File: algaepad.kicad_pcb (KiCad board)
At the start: 2 copper layers, 10.6 x 5.5 mm, 64 parts, among them SW1 SW_Push, SW10 SW_Push, SW11 SW_Push, SW12 SW_Push, SW13 SW_Push, SW14 SW_Push, SW15 SW_Push, SW16 SW_Push, SW17 SW_Push, SW18 SW_Push, SW19 SW_Push, SW2 SW_Push, SW20 SW_Push, SW21 SW_Push, SW22 SW_Push, SW23 SW_Push, SW24 SW_Push, SW25 SW_Push, SW26 SW_Push, SW27 SW_Push, SW28 SW_Push, SW29 SW_Push, SW3 SW_Push, SW30 SW_Push, SW31 SW_Push, SW32 SW_Push, SW4 SW_Push, SW5 SW_Push, SW6 SW_Push, SW7 SW_Push, SW8 SW_Push, SW9 SW_Push

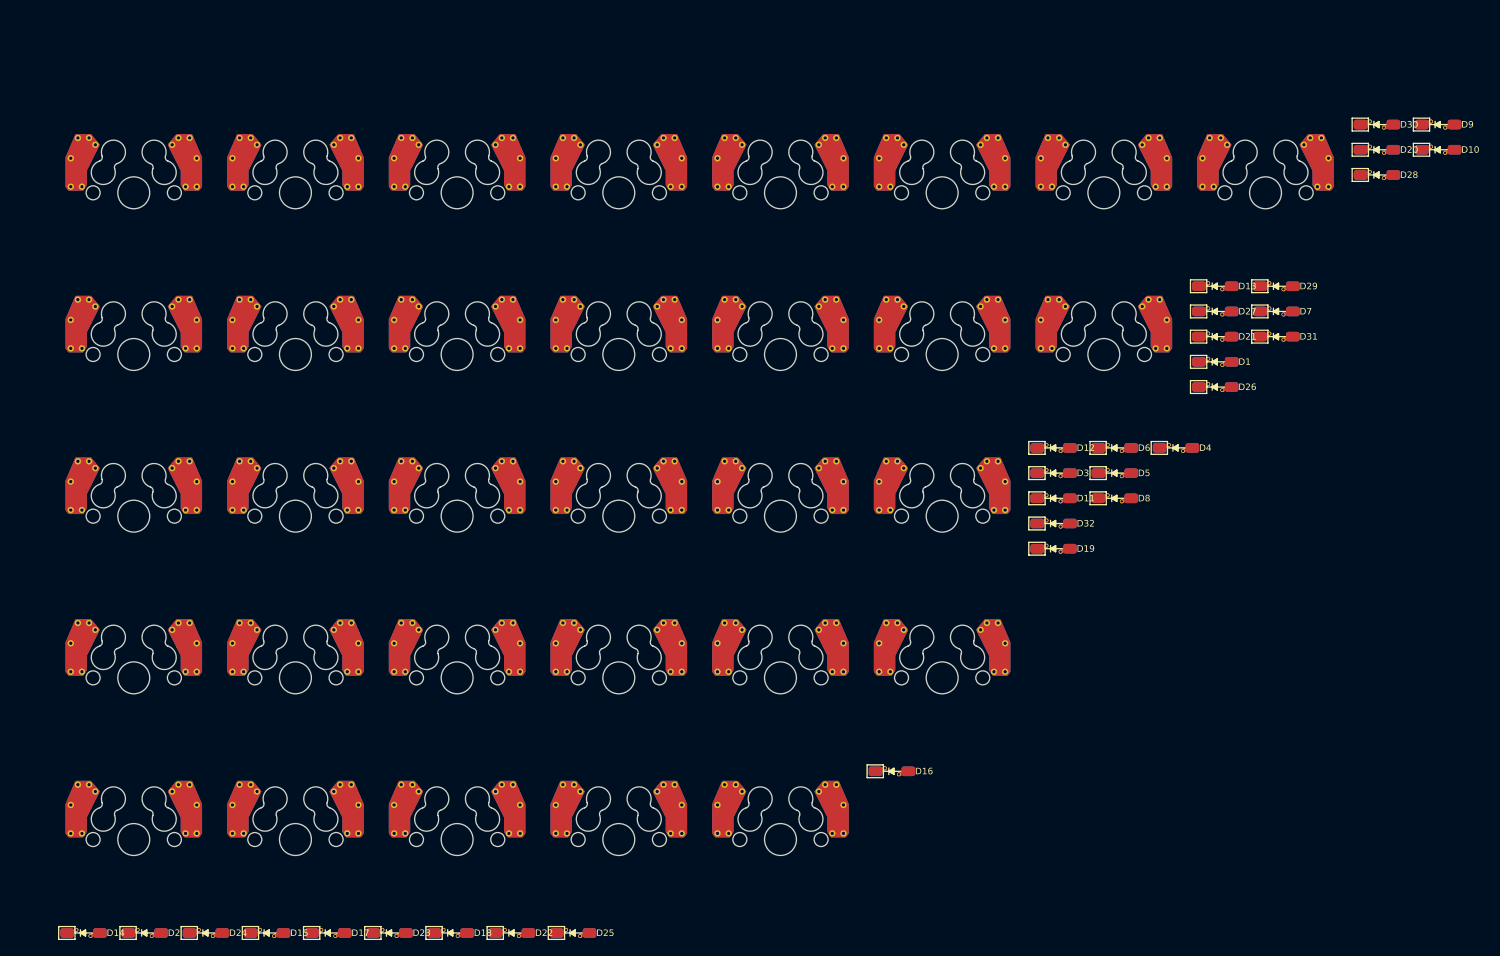
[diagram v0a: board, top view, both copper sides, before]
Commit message: start work in layout
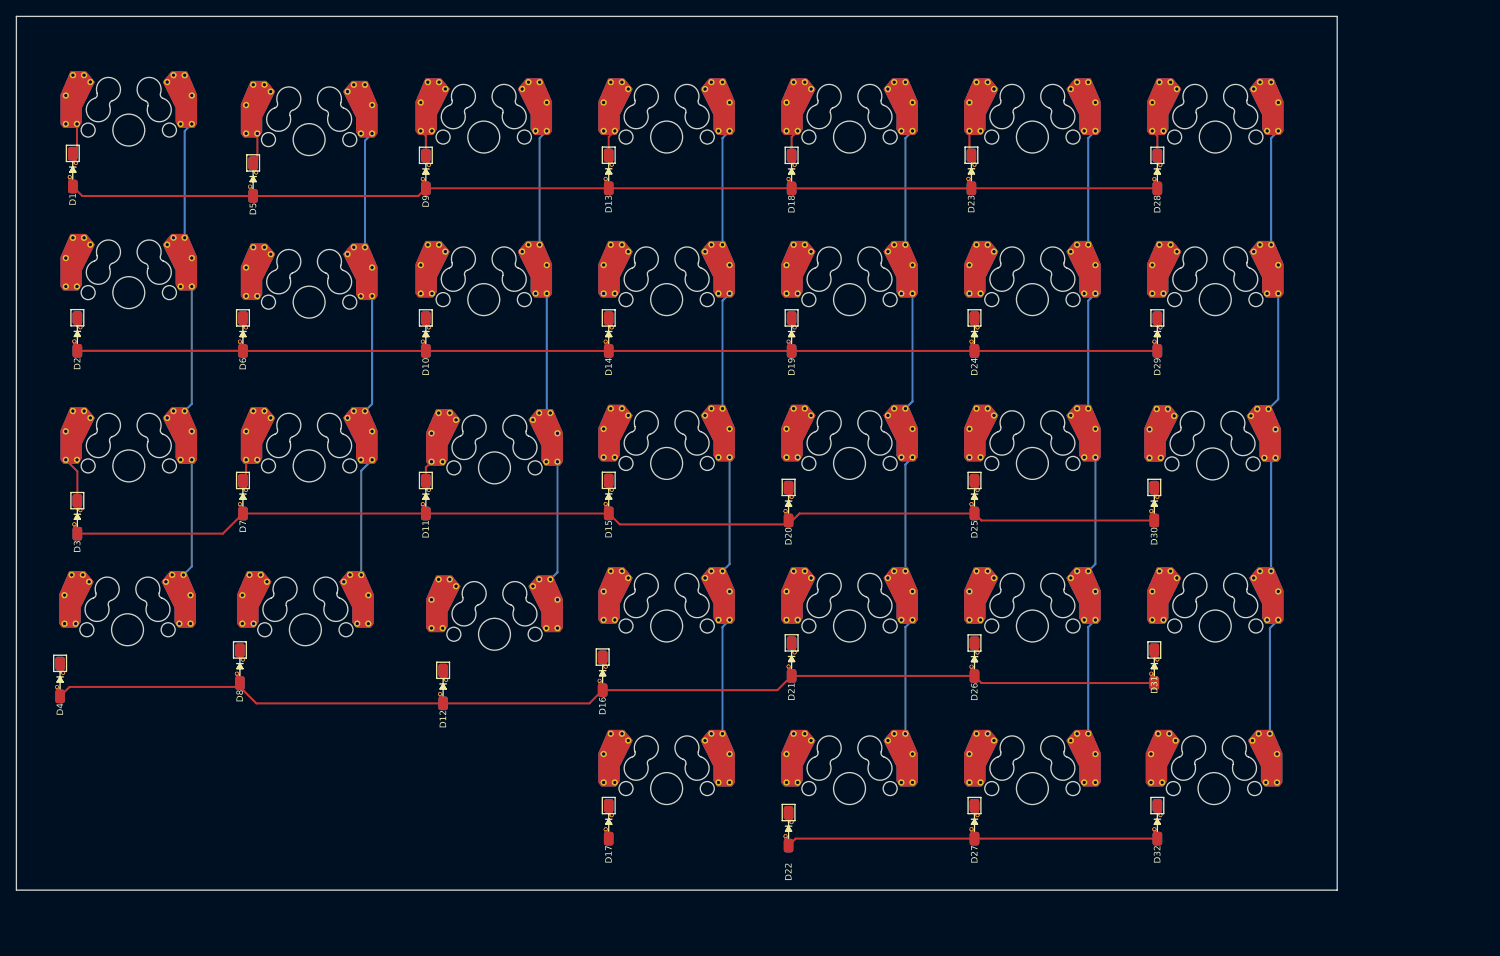
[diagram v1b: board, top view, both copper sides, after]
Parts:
- moved SW32 145.5 mm to (182.7, 111.8)
- moved D1 144.8 mm to (40.1, 34.4), turned to -90 degrees
- moved D4 142.5 mm to (38.5, 98.2), turned to -90 degrees
- moved D7 131.3 mm to (61.3, 75.3), turned to -90 degrees
- moved D10 128.6 mm to (84.2, 55.0), turned to -90 degrees
- moved D9 126.7 mm to (84.2, 34.7), turned to -90 degrees
- moved D3 122.2 mm to (40.6, 77.9), turned to -90 degrees
- moved SW24 121.9 mm to (160.0, 50.6)
- moved D24 121.8 mm to (152.8, 55.0), turned to -90 degrees
- moved D23 119.8 mm to (152.4, 34.7), turned to -90 degrees
- moved D5 113.8 mm to (62.6, 35.6), turned to -90 degrees
- moved D8 111.4 mm to (61.0, 96.5), turned to -90 degrees
- moved D6 109.9 mm to (61.3, 55.0), turned to -90 degrees
- moved SW1 106.4 mm to (47.1, 29.4)
- moved D18 104.2 mm to (129.9, 34.7), turned to -90 degrees
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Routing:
- net ROW4: track 0.00 -> 139.9 mm
- net ROW3: track 0.00 -> 137.2 mm
- net ROW1: track 0.00 -> 136.5 mm
- net ROW2: track 0.00 -> 135.0 mm
- net COL7: track 0.00 -> 58.6 mm
- net COL6: track 0.00 -> 58.5 mm
- net COL4: track 0.00 -> 58.5 mm
- net COL5: track 0.00 -> 58.5 mm
- net ROW5: track 0.00 -> 46.5 mm
- net COL1: track 0.00 -> 45.3 mm
- net COL3: track 0.00 -> 44.8 mm
- net COL2: track 0.00 -> 44.3 mm
- net Net-(D3-Pad1): track 0.00 -> 5.73 mm
- net Net-(D1-Pad1): track 0.00 -> 3.93 mm
- net Net-(D5-Pad1): track 0.00 -> 3.93 mm
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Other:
- board size 10.6 x 5.5 mm -> 165.1 x 109.2 mm
- rule pad_to_mask_clearance: 0 -> 0.05
